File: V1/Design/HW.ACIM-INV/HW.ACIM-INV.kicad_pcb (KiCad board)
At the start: 4 copper layers, 154 x 178.5 mm, 302 parts, among them J1 AC POWER INPUT, J2 FAN, J3 MOTOR, J4 MCDBG, J8 ENCODER, M1 560V/1.75kA, M2 560V/1.75kA, M3 560V/1.75kA, M4 470V/1.2kA, M5 470V/1.2kA, M6 470V/1.2kA, M7 470V/1.2kA, Q1 20V/1A, Q10 20V/1A, Q11 20V/1A, Q2 60V/265mA, Q3 20V/1A, Q4 20V/1A, Q5 20V/1A, Q6 20V/1A, Q7 60V/265mA, Q8 60V/265mA, Q9 60V/265mA, U1 IPM 600V/15A, U10 SMPS 12V±2%/0.8A, U11 2Mbit SRAM, U12 OP-1CH, U13 LDO 3.3V±0.5%/1A, U14 SMPS 15V±2%/0.6A, U15 I=±10A, U16 I=±10A, U17 LDO 5V±0.4%/250mA, U18 OP-1CH, U19 OP-1CH, U2 OP-1CH, U20 SMPS 5V±2%/1.2A, U3 ISEN 50mV/V, U4 CMP-1CH, U5 ISEN 50mV/V, U6 ISEN 50mV/V, U7 OP-1CH, U8 OP-1CH, U9 ISO6740

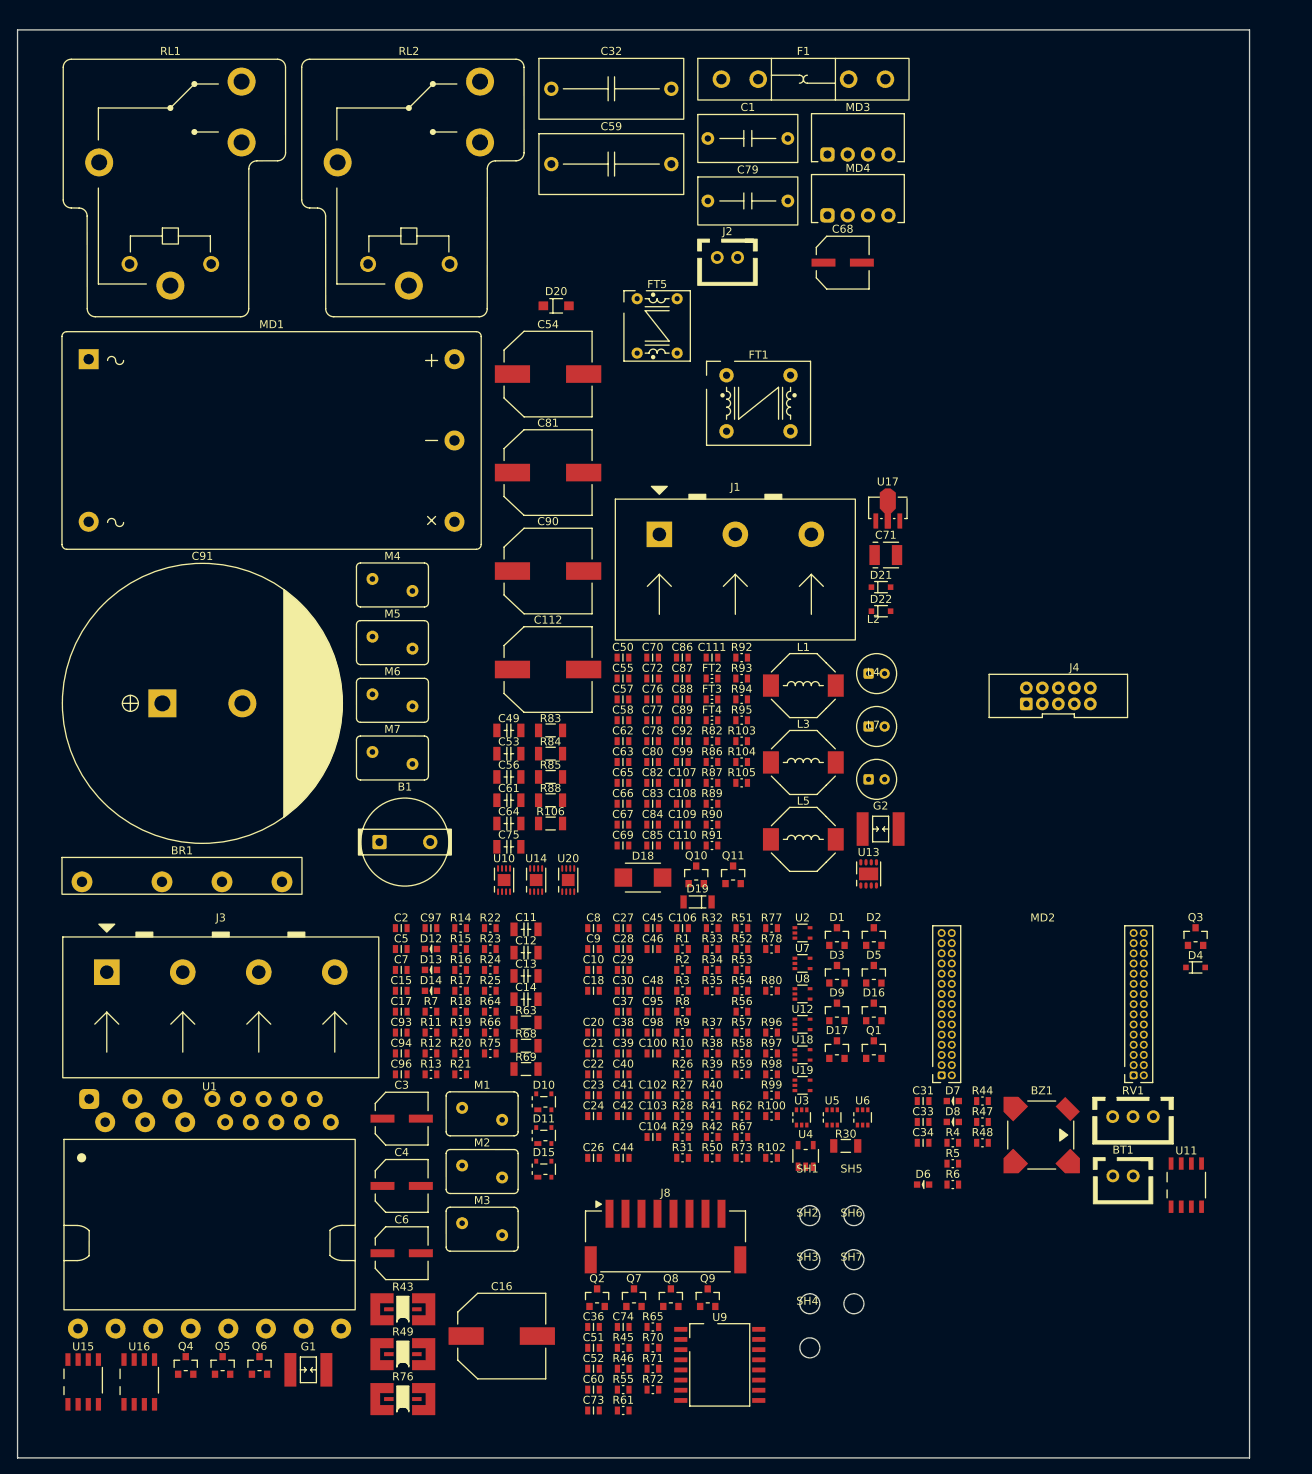
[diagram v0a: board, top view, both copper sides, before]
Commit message: V1 schematic update 17
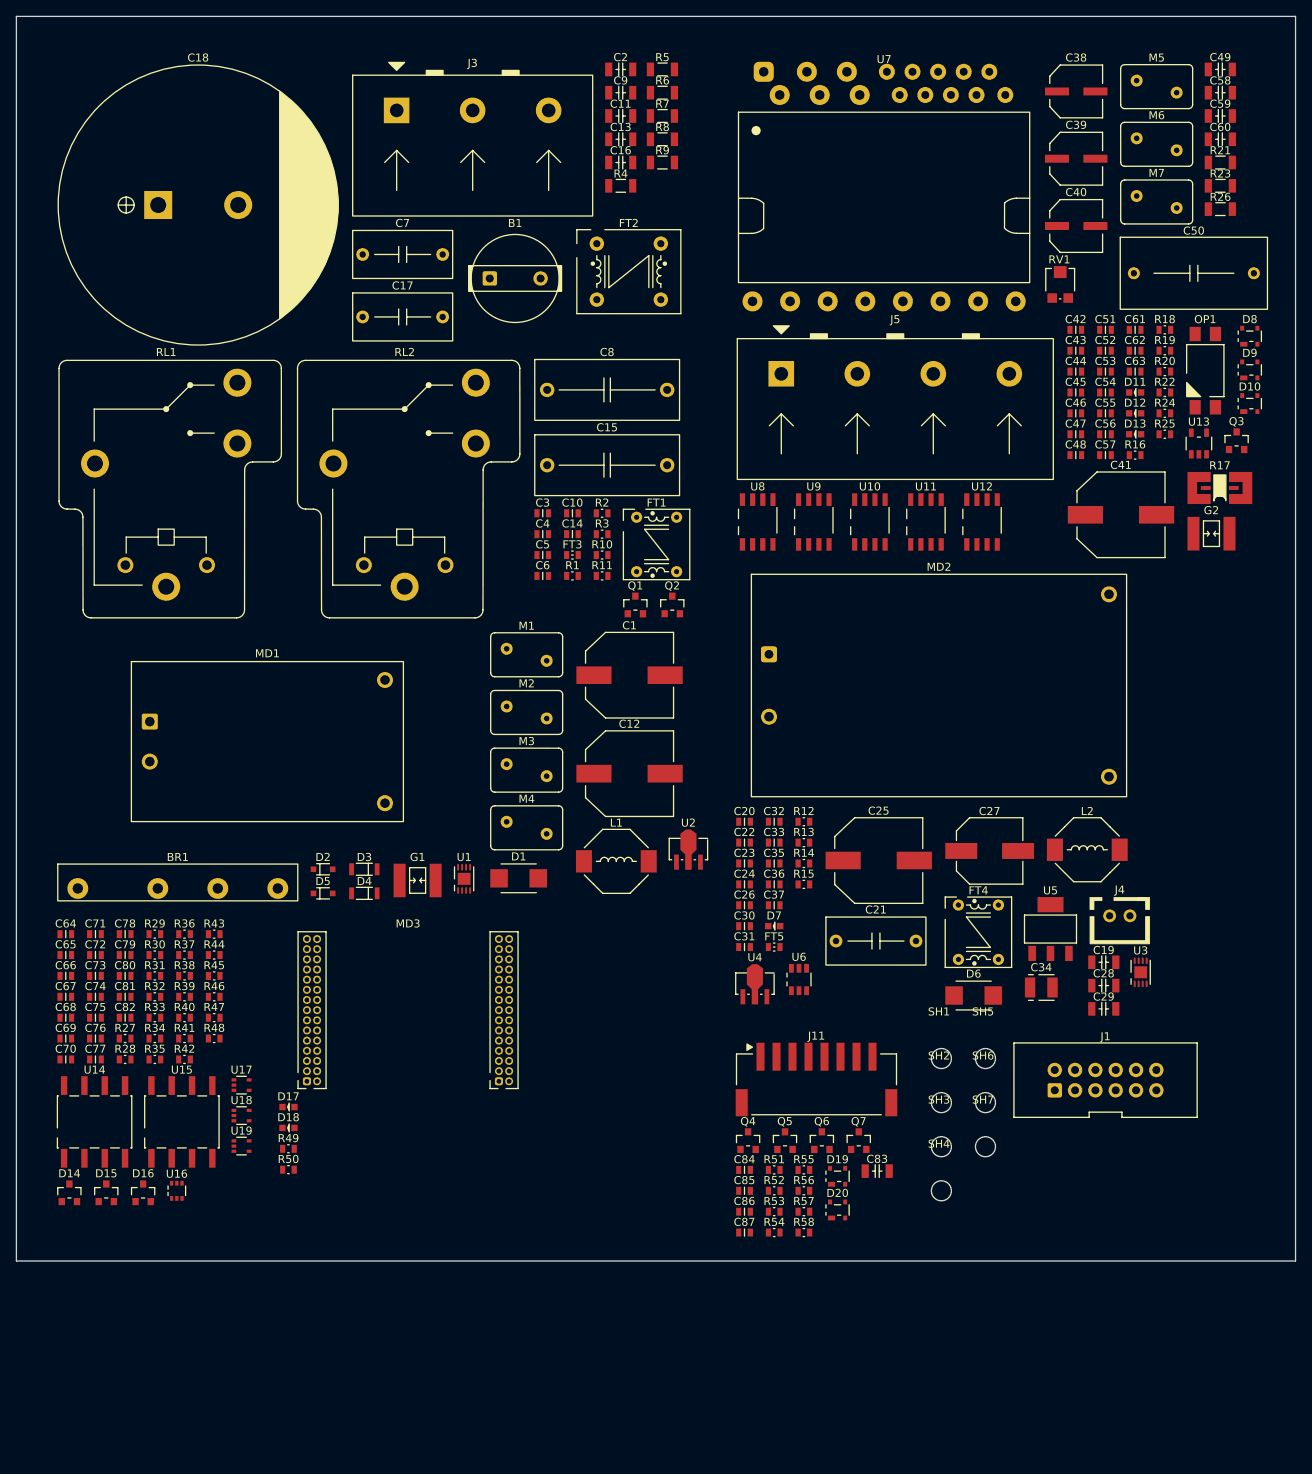
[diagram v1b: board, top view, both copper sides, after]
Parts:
- removed BT1: UBT, SAMPI:HDM-2x2.54-TH
- removed BZ1: BUZZER, SAMPI:SMT-0827-S-HT-R
- removed C100, C102, C103, C106, C94, C97, C98: 1nF, SAMPI:CAP0603
- removed C104, C109, C111, C89, C92, C93, C95, C96: 100nF, SAMPI:CAP0603
- removed C107: 10uF/35V, SAMPI:CAP0603
- removed C108, C88, C99: 10uF, SAMPI:CAP0603
- removed C110: 3.3nF, SAMPI:CAP0603
- removed C112, C90: 470uF/35V, SAMPI:CAP_ELEC-10.3x10.3-DIA10
- removed C91: 680uF/450V, SAMPI:ESMQ451VSN681MA50S
- removed D21, D22: 75V/150mA, SAMPI:SOD-323
- removed F1: 10A, SAMPI:01000056Z
- removed J2: FAN, SAMPI:HDM-2x2.54-TH
- removed J8: ENCODER, SAMPI:HDM1x8x2.0_SMA_RA
- removed L3: 22uH/1.5A, SAMPI:IND-8D43-8045
- removed L4, L7: 4.7uH/670mA, SAMPI:IND-R5-2MM-TH
- removed L5: 68uH/1A, SAMPI:IND-8D43-8045
- removed MD4: DC-DC 5V-5V/200mA, SAMPI:B1524S-1WR3
- removed Q10, Q11: 20V/1A, SAMPI:SOT23
- removed Q8, Q9: 60V/265mA, SAMPI:SOT23
- removed R100, R59, R78, R80: 10R, SAMPI:RES0603
- removed R102, R91, R95: 10K, SAMPI:RES0603
- removed R103, R62, R67, R73, R75, R82, R86, R92, R94, R96, R97, R98, R99: 100K, SAMPI:RES0603
- removed R104: 53.6K, 1%, SAMPI:RES0603
- removed R105, R90, R93: 10K, 1%, SAMPI:RES0603
- removed R106, R83, R84, R85, R88: 1M, SAMPI:RES1206
- removed R61, R65, R70, R71, R72: 4.3K, SAMPI:RES0603
- removed R63, R68, R69: 4.7R, SAMPI:RES1206
- removed R64, R66, R77: 1.1K, SAMPI:RES0603
- removed R76: 10mR/3W/1%, SAMPI:SHU2512
- removed R87: 180K, 1%, SAMPI:RES0603
- removed R89: 140K, 1%, SAMPI:RES0603
- removed U20: SMPS 5V±2%/1.2A, SAMPI:TDFN8_2x3_MCHP
- added C19: 10uF/35V, SAMPI:CAP1206, F.Cu at (150.5, 132.1)
- added C25: 470uF/35V, SAMPI:CAP_ELEC-10.3x10.3-DIA10, F.Cu at (122.4, 119.4)
- added C35: 100nF, SAMPI:CAP0603, F.Cu at (109.3, 119.8)
- added C43: 100nF, SAMPI:CAP0603, F.Cu at (147.0, 55.7)
- added C47: 10uF, SAMPI:CAP0603, F.Cu at (147.0, 66.1)
- added J11: ENCODER, SAMPI:HDM1x8x2.0_SMA_RA, F.Cu at (114.6, 146.7)
- added J5: MOTOR, SAMPI:TMB4_9.5, F.Cu at (124.5, 58.5)
- added OP1: OPTO-BJT-1CH, SAMPI:OPTO_SO4_7.6MM, F.Cu at (163.2, 58.1)
- added R36: 10R, 1%, SAMPI:RES0603, F.Cu at (35.6, 128.6)
- C1: value 100nF/400V -> 470uF/35V; footprint SAMPI:CAP_FILM_6.0x12.0x12.5-P10 -> SAMPI:CAP_ELEC-10.3x10.3-DIA10
- C10: value 1nF -> 100nF
- C12: value 100pF/2kV -> 470uF/25V; footprint SAMPI:CAP1206 -> SAMPI:CAP_ELEC-10.3x10.3-DIA10
- C14, C53: value 100pF/2kV -> 10uF; footprint SAMPI:CAP1206 -> SAMPI:CAP0603
- C15: value 22pF -> 1uF/400V; footprint SAMPI:CAP0603 -> SAMPI:ECWFE2W105
- C16: value 470uF -> 100pF/2kV; footprint SAMPI:CAP_ELEC-10.3x10.3-DIA10 -> SAMPI:CAP1206
- C17, C7: value 100nF -> 100nF/400V; footprint SAMPI:CAP0603 -> SAMPI:CAP_FILM_6.0x12.0x12.5-P10
- C18: value 1nF -> 680uF/450V; footprint SAMPI:CAP0603 -> SAMPI:ESMQ451VSN681MA50S
- C2, C28, C29: value 100nF -> 10uF/35V; footprint SAMPI:CAP0603 -> SAMPI:CAP1206
- C20, C46, C48: value 100nF -> 10uF
- C21: value 1nF -> 100nF/400V; footprint SAMPI:CAP0603 -> SAMPI:CAP_FILM_6.0x12.0x12.5-P10
- C23: value 100nF -> 3.3nF
- C27: value 100nF -> 470uF/16V; footprint SAMPI:CAP0603 -> SAMPI:CAP_ELEC-8.3x8.3-DIA8.0
- C3: value 47uF/35V -> 10uF; footprint SAMPI:CAP_ELEC-6.6x6.6-DIA6.3 -> SAMPI:CAP0603
- C30, C31, C37: value 1nF -> 10uF
- C32: value 1uF/400V -> 100nF; footprint SAMPI:ECWFE2W105 -> SAMPI:CAP0603
- C34: value 100nF -> 220uF/6.3V; footprint SAMPI:CAP0603 -> SAMPI:CAP1411
- C36, C51: value 22pF -> 100nF
- C38, C40: value 100nF -> 47uF/35V; footprint SAMPI:CAP0603 -> SAMPI:CAP_ELEC-6.6x6.6-DIA6.3
- C39: value 1nF -> 47uF/35V; footprint SAMPI:CAP0603 -> SAMPI:CAP_ELEC-6.6x6.6-DIA6.3
- C4, C68: value 47uF/35V -> 100nF; footprint SAMPI:CAP_ELEC-6.6x6.6-DIA6.3 -> SAMPI:CAP0603
- C41: value 100nF -> 470uF/25V; footprint SAMPI:CAP0603 -> SAMPI:CAP_ELEC-10.3x10.3-DIA10
- C50: value 100nF -> 470nF/630V; footprint SAMPI:CAP0603 -> SAMPI:FCAP-15MM
- C52: value 22pF -> 1nF
- C54: value 470uF/35V -> 10uF; footprint SAMPI:CAP_ELEC-10.3x10.3-DIA10 -> SAMPI:CAP0603
- C56, C61: value 100pF/2kV -> 100nF; footprint SAMPI:CAP1206 -> SAMPI:CAP0603
- C57, C74: value 10uF -> 1nF
- C58, C9: value 100nF -> 100pF/2kV; footprint SAMPI:CAP0603 -> SAMPI:CAP1206
- C59: value 1uF/400V -> 100pF/2kV; footprint SAMPI:ECWFE2W105 -> SAMPI:CAP1206
- C6: value 47uF/35V -> 3.3nF; footprint SAMPI:CAP_ELEC-6.6x6.6-DIA6.3 -> SAMPI:CAP0603
- C60: value 22pF -> 100pF/2kV; footprint SAMPI:CAP0603 -> SAMPI:CAP1206
- C62: value 10uF/35V -> 100nF
- C64, C75: value 100pF/2kV -> 1nF; footprint SAMPI:CAP1206 -> SAMPI:CAP0603
- C65, C76, C77, C78: value 100nF -> 1nF
- C66: value 3.3nF -> 100nF
- C70, C82: value 10uF/35V -> 1nF
- C71: value 220uF/6.3V -> 1nF; footprint SAMPI:CAP1411 -> SAMPI:CAP0603
- C72, C73, C80: value 10uF -> 100nF
- C79: value 100nF/400V -> 100nF; footprint SAMPI:CAP_FILM_6.0x12.0x12.5-P10 -> SAMPI:CAP0603
- C8: value 1nF -> 1uF/400V; footprint SAMPI:CAP0603 -> SAMPI:ECWFE2W105
- C81: value 470uF/35V -> 1nF; footprint SAMPI:CAP_ELEC-10.3x10.3-DIA10 -> SAMPI:CAP0603
- C83: value 10uF -> 10uF/35V; footprint SAMPI:CAP0603 -> SAMPI:CAP1206
- C84: value 100nF -> 22pF
- C85: value 3.3nF -> 22pF
- D1: value GP DIODE -> 24V; footprint SAMPI:SOT23 -> SAMPI:DO-214AA-12
- D10: value TVS 5.5V 3-CH -> TVS 5.5V
- D11: value TVS 5.5V 3-CH -> PV; footprint SAMPI:SOT143B_NEXT -> SAMPI:LED0603
- D12: value PU -> PW
- D13: value PV -> PU
- D14: value PW -> GP DIODE; footprint SAMPI:LED0603 -> SAMPI:SOT23
- D15: value TVS 5.5V 3-CH -> GP DIODE; footprint SAMPI:SOT143B_NEXT -> SAMPI:SOT23
- D17: value GP DIODE -> ERR; footprint SAMPI:SOT23 -> SAMPI:LED0603
- D18: value 24V -> RUN; footprint SAMPI:DO-214AA-12 -> SAMPI:LED0603
- D19: value 24V -> TVS 5.5V; footprint SAMPI:SOD-80C_DO-213AC -> SAMPI:SOT143B_NEXT
- D2, D5: value GP DIODE -> 75V/150mA; footprint SAMPI:SOT23 -> SAMPI:SOD-323
- D20: value 5.1V -> TVS 5.5V; footprint Liem:SOD-123 -> SAMPI:SOT143B_NEXT
- D3: value GP DIODE -> 6V2; footprint SAMPI:SOT23 -> SAMPI:SOD80C-LL34
- D4: value 75V/150mA -> 6V2; footprint SAMPI:SOD-323 -> SAMPI:SOD80C-LL34
- D6: value ERR -> 24V; footprint SAMPI:LED0603 -> SAMPI:DO-214AA-12
- D7: value RUN -> PWR
- D8: value PWR -> TVS 5.5V; footprint SAMPI:LED0603 -> SAMPI:SOT143B_NEXT
- D9: value GP DIODE -> TVS 5.5V; footprint SAMPI:SOT23 -> SAMPI:SOT143B_NEXT
- FT1: value 5mH/2.5A -> 15mH/500mA; footprint SAMPI:IND-SQ1010 -> SAMPI:EE8.3
- FT2: value 120R@100MHz -> 5mH/2.5A; footprint SAMPI:FT0603 -> SAMPI:IND-SQ1010
- FT4: value 120R@100MHz -> 15mH/500mA; footprint SAMPI:FT0603 -> SAMPI:EE8.3
- FT5: value 15mH/500mA -> 120R@100MHz; footprint SAMPI:EE8.3 -> SAMPI:FT0603
- J1: value AC POWER INPUT -> MCDBG; footprint SAMPI:TMB3_9.5 -> SAMPI:IDC-2x6x2.54MM_TH
- J3: value MOTOR -> AC POWER INPUT; footprint SAMPI:TMB4_9.5 -> SAMPI:TMB3_9.5
- J4: value MCDBG -> FAN; footprint SAMPI:IDC-2x5x2MM-TH -> SAMPI:HDM-2x2.54-TH
- L1: value 56uH/1A -> 68uH/1A
- L2: value 4.7uH/670mA -> 56uH/1A; footprint SAMPI:IND-R5-2MM-TH -> SAMPI:IND-8D43-8045
- M1, M2, M3: value 560V/1.75kA -> 470V/1.2kA
- M5, M6, M7: value 470V/1.2kA -> 560V/1.75kA
- MD1: value AC-DC 24V±2%/10W -> 24V±2%/3W; footprint SAMPI:LD10-23BxxR2-RC -> SAMPI:HLK-PMxx
- MD2: value ACIM-MCU -> 24V±2%/10W; footprint SAMPI:HW.ACIM-MCU -> SAMPI:HLK-10M
- MD3: value DC-DC 15V/24V-24V/42mA -> ACIM-MCU; footprint SAMPI:B1524S-1WR3 -> SAMPI:HW.ACIM-MCU
- Q2: value 60V/265mA -> 20V/1A
- Q4, Q5, Q6: value 20V/1A -> 60V/265mA
- R1: value 10R -> 10K
- R10, R11, R22: value 1.1K -> 10K
- R12, R16: value 100K -> 10K
- R13: value 1.1K -> 140K, 1%
- R14: value 1.1K -> 10K, 1%
- R15, R19, R20: value 1.1K -> 1K
- R17: value 100K -> 10mR/3W/1%; footprint SAMPI:RES0603 -> SAMPI:SHU2512
- R18, R24: value 100K -> 1K
- R2: value 10R -> 191K, 1%
- R21: value 1.1K -> 4.7R; footprint SAMPI:RES0603 -> SAMPI:RES1206
- R23, R26: value 100K -> 4.7R; footprint SAMPI:RES0603 -> SAMPI:RES1206
- R25: value 100K -> 1.2M
- R27: value 10R -> 100K, 1%
- R28: value 100K -> 100K, 1%
- R29, R44: value 1.1K -> 100K, 1%
- R3: value 5.2K -> 10K, 1%
- R30: value 1M -> 1.1K, 1%; footprint SAMPI:RES1206 -> SAMPI:RES0603
- R31: value 470K -> 10R, 1%
- R32, R41: value 10R -> 10R, 1%
- R33, R47: value 1.1K -> 10R, 1%
- R34, R35: value 100K -> 10R, 1%
- R37: value 100K -> 10K, 1%
- R38: value 10R -> 10K, 1%
- R39: value 1.1K -> 4.99K, 1%
- R4: value 10R -> 1M; footprint SAMPI:RES0603 -> SAMPI:RES1206
- R40: value 10R -> 4.99K, 1%
- R42: value 5.2K -> 10R, 1%
- R43: value 10mR/3W/1% -> 100K, 1%; footprint SAMPI:SHU2512 -> SAMPI:RES0603
- R45, R46: value 4.3K -> 100K, 1%
- R48: value 10K -> 10R, 1%
- R49: value 10mR/3W/1% -> 1K; footprint SAMPI:SHU2512 -> SAMPI:RES0603
- R5, R7: value 1.1K -> 1M; footprint SAMPI:RES0603 -> SAMPI:RES1206
- R50: value 10R -> 1K
- R51, R52: value 10R -> 2.2K
- R53, R56, R57: value 100K -> 2.2K
- R54: value 10K -> 2.2K
- R55: value 4.3K -> 2.2K
- R58: value 1.1K -> 2.2K
- R6, R8, R9: value 100K -> 1M; footprint SAMPI:RES0603 -> SAMPI:RES1206
- RV1: value 10K -> 20K; footprint Liem:HDM-3x2.54-TH -> SAMPI:TC33X-2
- U1: value IPM 600V/15A -> SMPS 16V±2%/0.6A; footprint SAMPI:CIPOS-MINI -> SAMPI:TDFN8_2x3_MCHP
- U10: value SMPS 12V±2%/0.8A -> DIGI ISO; footprint SAMPI:TDFN8_2x3_MCHP -> SAMPI:SOIC8_ALL
- U11: value 2Mbit SRAM -> I=±10A; footprint SAMPI:SOIC8_3.9_MCHP -> SAMPI:SOIC8_ALL
- U12: value OP-1CH -> I=±10A; footprint SAMPI:SOT353 -> SAMPI:SOIC8_ALL
- U13: value LDO 3.3V±0.5%/1A -> CMP-1CH; footprint SAMPI:DFN8_3x3_MCHP -> SAMPI:SOT25_DIODES
- U14: value SMPS 15V±2%/0.6A -> ISO OPAMP 1-CH; footprint SAMPI:TDFN8_2x3_MCHP -> SAMPI:SOP8-2.54
- U15: value I=±10A -> ISO OPAMP 1-CH; footprint SAMPI:SOIC8_ALL -> SAMPI:SOP8-2.54
- U16: value I=±10A -> ISEN 50mV/V; footprint SAMPI:SOIC8_ALL -> SAMPI:SOT363
- U17: value LDO 5V±0.4%/250mA -> OP-1CH; footprint SAMPI:SOT-89 -> SAMPI:SOT353
- U2: value OP-1CH -> LDO 5V±1%; footprint SAMPI:SOT353 -> SAMPI:SOT-89
- U3: value ISEN 50mV/V -> SMPS 12V±2%/0.8A; footprint SAMPI:SOT363 -> SAMPI:TDFN8_2x3_MCHP
- U4: value CMP-1CH -> LDO 5V±1%; footprint SAMPI:SOT25_DIODES -> SAMPI:SOT-89
- U5: value ISEN 50mV/V -> LDO 3V3±2%; footprint SAMPI:SOT363 -> SAMPI:SOT-223-3
- U6: value ISEN 50mV/V -> LDO 3.3V±0.1%/20mA; footprint SAMPI:SOT363 -> SAMPI:SOT-23-6_MCHP
- U7: value OP-1CH -> IPM 600V/15A; footprint SAMPI:SOT353 -> SAMPI:CIPOS-MINI
- U8: value OP-1CH -> DIGI ISO; footprint SAMPI:SOT353 -> SAMPI:SOIC8_ALL
- U9: value ISO6740 -> DIGI ISO; footprint SAMPI:SOIC16-W -> SAMPI:SOIC8_ALL
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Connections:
- B1 pad 1: Net-(RL1-NC) -> Net-(RL2-NC)
- C10 pad 1: AGND -> GND_INV
- C10 pad 2: /MCU/MC_ALT_IU_SEN -> +16V_INV
- C11 pad 2: /Inverter/MC_UW -> CHASSIS
- C13 pad 1: /Inverter/MC_UU -> AC1
- C13 pad 2: Net-(C13-Pad2) -> CHASSIS
- C14 pad 1: VDC -> GND_INV
- C14 pad 2: PGND -> +5V_INV
- C15 pad 1: AGND -> AC2
- C15 pad 2: /Inverter/MC_TEMP_SEN -> AC1
- C17 pad 1: +15V -> PGND
- C17 pad 2: GND -> VDC
- C2 pad 1: Net-(U1-VBU) -> GND_INV
- C2 pad 2: Net-(U1-VSU) -> +24V_INV
- C20 pad 1: /MCU/MC_UU_DIV -> GND_MCU
- C20 pad 2: AGND -> Net-(U3-VCC)
- C21 pad 1: GND -> Net-(MD2-ACN)
- C21 pad 2: /MCU/~{MC_PWM_FLT} -> Net-(MD2-ACL)
- C22 pad 1: AGND -> Net-(U3-SW)
- C22 pad 2: Net-(C22-Pad2) -> Net-(U3-BOOST)
- C23 pad 1: Net-(D2-COM) -> Net-(U3-VFB)
- C23 pad 2: AGND -> +12V_MCU
- C24 pad 1: AGND -> GND_MCU
- C24 pad 2: AVDD -> +24V_MCU
- C26 pad 1: /MCU/MC_UV_DIV -> GND_MCU
- C26 pad 2: AGND -> +12V_MCU
- C28 pad 1: Net-(D3-COM) -> GND_MCU
- C28 pad 2: AGND -> +12V_MCU
- C29 pad 1: GND -> GND_MCU
- C29 pad 2: VREF -> +12V_MCU
- C30 pad 1: AGND -> GND_MCU
- C30 pad 2: /MCU/MC_IV_SEN -> +5V_MCU
- C31 pad 1: AGND -> GND_MCU
- C31 pad 2: /MCU/MC_VR_DIV -> +5V_MCU
- C32 pad 1: Net-(C32-Pad1) -> GND_MCU
- C32 pad 2: Net-(C32-Pad2) -> +3V3_MCU
- C33 pad 1: GND -> GND_MCU
- C33 pad 2: /MCU/~{BT_UBT} -> +5V_MCU
- C36 pad 1: GND -> GND_ADC
- C36 pad 2: /ENCODER/ENC_HOME -> +3V3_ADC
- C37 pad 1: Net-(D9-COM) -> GND_ADC
- C37 pad 2: Net-(D9-A1) -> +3V3_ADC
- C42 pad 1: AGND -> +16V_INV
- C42 pad 2: AVDD -> GND_INV
- C44 pad 1: /MCU/MC_UW_DIV -> Net-(U7-VBV)
- C44 pad 2: AGND -> Net-(U7-VSV)
- C45 pad 1: Net-(D17-COM) -> Net-(U7-VBW)
- C45 pad 2: AGND -> Net-(U7-VSW)
- C46 pad 1: AGND -> GND_INV
- C46 pad 2: AVDD -> +5V_INV
- C48 pad 1: /MCU/MC_UDC_DIV -> GND_INV
- C48 pad 2: AGND -> +5V_INV
- C49 pad 1: Net-(C32-Pad1) -> VDC
- C49 pad 2: CHASSIS -> PGND
- C5 pad 1: Net-(U1-VBV) -> Net-(U1-SW)
- C5 pad 2: Net-(U1-VSV) -> Net-(U1-BOOST)
- C50 pad 1: GND -> VDC
- C50 pad 2: +24V -> PGND
- C51 pad 1: GND -> GND_MCU
- C51 pad 2: /ENCODER/ENC_A -> +5V_MCU
- C52 pad 1: GND -> GND_MCU
- C52 pad 2: /ENCODER/ENC_B -> Net-(U11-FILTER)
- C53 pad 1: Net-(C32-Pad2) -> GND_MCU
- C53 pad 2: CHASSIS -> +3V3_MCU
- C55 pad 1: GND -> GND_MCU
- C55 pad 2: Net-(MD4-VI+) -> +3V3_MCU
- C56 pad 1: AC1 -> GND_MCU
- C56 pad 2: CHASSIS -> +5V_MCU
- C57 pad 1: GND -> GND_MCU
- C57 pad 2: Net-(U10-VCC) -> Net-(U12-FILTER)
- C58 pad 1: GND -> /INVERTER/MC_U
- C58 pad 2: +15V -> Net-(C58-Pad2)
- C59 pad 1: AC2 -> Net-(C59-Pad1)
- C59 pad 2: AC1 -> /INVERTER/MC_V
- C60 pad 1: GND -> /INVERTER/MC_W
- C60 pad 2: /ENCODER/ENC_INDEX -> Net-(C60-Pad2)
- C61 pad 1: AC2 -> GND_INV
- C61 pad 2: CHASSIS -> +5V_INV
- C62 pad 1: GND -> GND_INV
- C62 pad 2: Net-(MD3-VI+) -> Net-(RV1-WIPER)
- C63 pad 1: Net-(U10-SW) -> GND_INV
- C63 pad 2: Net-(U10-BOOST) -> /INVERTER/IPM_TEMP_SEN
- C64 pad 1: GND -> Net-(D15-COM)
- C64 pad 2: GND1 -> Net-(D15-A1)
- C65 pad 1: GND -> Net-(D16-COM)
- C65 pad 2: +5V -> Net-(D16-A1)
- C66 pad 1: Net-(U10-VFB) -> +5V_INV
- C66 pad 2: +12V -> GND_INV
- C67 pad 1: GND1 -> +5V_INV
- C67 pad 2: +24V_ISO -> GND_INV
- C69 pad 1: GND -> +5V_MCU
- C69 pad 2: +12V -> GND_MCU
- C7 pad 1: Net-(U1-VBW) -> Net-(MD1-ACN)
- C7 pad 2: Net-(U1-VSW) -> Net-(MD1-ACL)
- C70 pad 1: GND -> Net-(U16-IN-)
- C70 pad 2: +24V -> Net-(U16-IN+)
- C72 pad 1: GND -> GND_MCU
- C72 pad 2: +5V -> +5V_MCU
- C73 pad 1: GND_ISO -> GND_MCU
- C73 pad 2: +5V_ISO -> +5V_MCU
- C74 pad 1: GND -> GND_ADC
- C74 pad 2: +3V3 -> /MCU/MC_UDC_DIV
- C75 pad 1: GND -> GND_ADC
- C75 pad 2: GND1 -> Net-(U16-OUT)
- C76 pad 1: GND1 -> GND_ADC
- C76 pad 2: +5V_ISO -> /MCU/MC_IDC_SEN
- C77 pad 1: GND -> GND_MCU
- C77 pad 2: Net-(U13-CDELAY) -> Net-(U18-IN+)
- C78 pad 1: GND -> GND_MCU
- C78 pad 2: +3V3 -> Net-(U19-IN+)
- C79 pad 1: PGND -> GND_MCU
- C79 pad 2: VDC -> +5V_MCU
- C8 pad 1: Net-(D1-COM) -> Net-(C8-Pad1)
- C8 pad 2: Net-(D1-A1) -> Net-(C11-Pad1)
- C80 pad 1: GND1 -> GND_MCU
- C80 pad 2: +5V_ISO -> +5V_MCU
- C82 pad 1: GND -> GND_ADC
- C82 pad 2: +24V -> /MCU/MC_IV_SEN
- C83 pad 1: GND -> GND_MCU
- C83 pad 2: Net-(U14-VCC) -> /ENCODER/V_ENC
- C84 pad 1: Net-(U14-SW) -> GND_MCU
- C84 pad 2: Net-(U14-BOOST) -> /ENCODER/ENC_HOME
- C85 pad 1: Net-(U14-VFB) -> GND_MCU
- C85 pad 2: +15V -> /ENCODER/ENC_INDEX
- C86 pad 1: GND -> GND_MCU
- C86 pad 2: +3V3 -> /ENCODER/ENC_B
- C87 pad 1: AGND -> GND_MCU
- C87 pad 2: AVDD -> /ENCODER/ENC_A
- C9 pad 1: GND -> Net-(C8-Pad1)
- C9 pad 2: VREF -> CHASSIS
- D1 pad 1: Net-(D1-A1) -> GND_INV
- D1 pad 2: Net-(D1-A1) -> +24V_INV
- D10 pad 1: GND -> GND_INV
- D10 pad 2: /Inverter/MC_PWM_UH -> /INVERTER/IPM_PWM_WH
- D10 pad 3: /Inverter/MC_PWM_VH -> /INVERTER/IPM_PWM_WL
- D10 pad 4: +3V3 -> +5V_INV
- D12 pad K: Net-(Q4-D) -> GND_MCU
- D13 pad K: Net-(Q5-D) -> GND_MCU
- D15 pad 1: GND -> Net-(D15-A1)
- D15 pad 2: /Inverter/MC_PWM_WL -> Net-(D15-A1)
- D15 pad 3: /Inverter/MC_PWM_WH -> Net-(D15-COM)
- D16 pad 1: AGND -> Net-(D16-A1)
- D16 pad 2: AVDD -> Net-(D16-A1)
- D4 pad A: Net-(BZ1-V-) -> Net-(Q2-D)
- D4 pad K: +5V -> Net-(RL2-COIL1)
- D7 pad A: /MCU/IND_RUN -> Net-(D7-PadA)
- D7 pad K: Net-(D7-PadK) -> GND_MCU
- D9 pad 1: Net-(D9-A1) -> GND_INV
- D9 pad 2: Net-(D9-A1) -> /INVERTER/IPM_PWM_VH
- D9 pad 3: Net-(D9-COM) -> /INVERTER/IPM_PWM_VL
- FT1 pad 1: Net-(C32-Pad1) -> AC2
- FT1 pad 2: AC2 -> Net-(MD1-ACN)
- FT1 pad 3: Net-(C32-Pad2) -> AC1
- FT1 pad 4: AC1 -> Net-(MD1-ACL)
- FT2 pad 1: AGND -> Net-(C8-Pad1)
- FT2 pad 2: GND -> AC2
- FT3 pad 1: GND -> GND_INV
- FT4 pad 1: +3V3 -> AC2
- FT4 pad 2: AVDD -> Net-(MD2-ACN)
- FT5 pad 1: AC2 -> GND_MCU
- FT5 pad 2: Net-(MD1-ACN) -> GND_ADC
- G2 pad 1: CHASSIS -> Net-(G2-Pad1)
- G2 pad 2: Net-(G2-Pad2) -> CHASSIS
- J1 pad 1: CHASSIS -> /MCU/DB_TXD
- J1 pad 2: Net-(C32-Pad1) -> /MCU/~{MCLR}
- J1 pad 3: Net-(F1-Pad1) -> /MCU/DB_RXD
- J3 pad 1: Net-(G1-Pad2) -> CHASSIS
- J3 pad 2: /Inverter/MC_UV -> Net-(C8-Pad1)
- J3 pad 3: /Inverter/MC_UW -> Net-(C11-Pad1)
- J4 pad 1: /MCU/DV_TXD -> +12V_MCU
- J4 pad 2: /MCU/~{MCLR} -> GND
- L1 pad 1: Net-(U10-SW) -> Net-(U1-SW)
- L1 pad 2: +12V -> +16V_INV
- L2 pad 1: +15V -> Net-(U3-SW)
- L2 pad 2: Net-(MD3-VI+) -> +12V_MCU
- M1 pad 1: Net-(G1-Pad2) -> Net-(C8-Pad1)
- M1 pad 2: /Inverter/MC_UV -> Net-(C11-Pad1)
- M2 pad 2: /Inverter/MC_UW -> Net-(C8-Pad1)
- M3 pad 2: /Inverter/MC_UU -> Net-(C11-Pad1)
- M4 pad 1: Net-(C32-Pad1) -> AC2
- M4 pad 2: Net-(C32-Pad2) -> AC1
- M5 pad 1: Net-(G2-Pad2) -> Net-(G2-Pad1)
- M5 pad 2: Net-(C32-Pad1) -> /INVERTER/MC_U
- M6 pad 1: Net-(G2-Pad2) -> Net-(G2-Pad1)
- M6 pad 2: Net-(C32-Pad2) -> /INVERTER/MC_V
- M7 pad 1: AC2 -> Net-(G2-Pad1)
- M7 pad 2: AC1 -> /INVERTER/MC_W
- MD1 pad 3: unconnected-(MD1-NC-Pad3) -> GND_INV
- MD1 pad 4: GND -> +24V_INV
- Q1 pad 1: /MCU/~{MC_PWM_FLT} -> /INVERTER POWER/PWR_RELAY
- Q1 pad 2: GND -> GND_MCU
- Q1 pad 3: /Inverter/MC_PWM_FLT -> Net-(Q1-D)
- Q2 pad 1: +5V_ISO -> /INVERTER POWER/~{DEV_RELAY}
- Q2 pad 2: Net-(Q2-S) -> GND_MCU
- Q2 pad 3: /ENCODER/HOME -> Net-(Q2-D)
- Q3 pad 1: /MCU/IND_ERR -> /INVERTER/IPM_PWM_FLT
- Q3 pad 2: GND -> GND_INV
- Q3 pad 3: Net-(BZ1-V-) -> Net-(OP1-K)
- Q4 pad 1: /Inverter/IPM_PWM_UL -> +3V3_MCU
- Q4 pad 2: GND -> /ENCODER/ENC_HOME
- Q4 pad 3: Net-(Q4-D) -> /ENCODER/HOME
- Q5 pad 1: /Inverter/IPM_PWM_VL -> +3V3_MCU
- Q5 pad 2: GND -> /ENCODER/ENC_INDEX
- Q5 pad 3: Net-(Q5-D) -> /ENCODER/INDEX
- Q6 pad 1: /Inverter/IPM_PWM_WL -> +3V3_MCU
- Q6 pad 2: GND -> /ENCODER/ENC_B
- Q6 pad 3: Net-(Q6-D) -> /ENCODER/PULSE_B
- Q7 pad 1: +5V_ISO -> +3V3_MCU
- Q7 pad 2: Net-(Q7-S) -> /ENCODER/ENC_A
- Q7 pad 3: /ENCODER/INDEX -> /ENCODER/PULSE_A
- R1 pad 1: Net-(D1-A1) -> Net-(U1-EN)
- R1 pad 2: /Inverter/MC_IU_SEN_P -> +24V_INV
- R10 pad 1: Net-(U4-VIN-) -> /INVERTER POWER/PWR_RELAY
- R10 pad 2: /MCU/MC_IDC_SEN -> GND_MCU
- R11 pad 1: Net-(U1-VFO) -> /INVERTER POWER/~{DEV_RELAY}
- R11 pad 2: /Inverter/MC_TEMP_SEN -> GND_MCU
- R12 pad 1: AVDD -> Net-(U3-EN)
- R12 pad 2: Net-(U1-VFO) -> +24V_MCU
- R13 pad 1: /Inverter/IPM_PWM_UH -> Net-(U3-VFB)
- R13 pad 2: /Inverter/MC_PWM_UH -> +12V_MCU
- R14 pad 1: /Inverter/IPM_PWM_VH -> GND_MCU
- R14 pad 2: /Inverter/MC_PWM_VH -> Net-(U3-VFB)
- R15 pad 1: /Inverter/IPM_PWM_WH -> +3V3_MCU
- R15 pad 2: /Inverter/MC_PWM_WH -> Net-(D7-PadA)
- R16 pad 1: GND -> +5V_INV
- R16 pad 2: /Inverter/IPM_PWM_WH -> /INVERTER/IPM_TEMP_SEN
- R17 pad 1: GND -> PGND
- R17 pad 2: /Inverter/IPM_PWM_VH -> Net-(U7-NU)
- R18 pad 1: GND -> Net-(D13-PadA)
- R18 pad 2: /Inverter/IPM_PWM_UH -> /INVERTER/MC_PWM_UH
- R19 pad 1: /Inverter/IPM_PWM_UL -> Net-(D11-PadA)
- R19 pad 2: /Inverter/MC_PWM_UL -> /INVERTER/MC_PWM_VH
- R2 pad 1: Net-(D1-COM) -> Net-(U1-VFB)
- R2 pad 2: /Inverter/MC_IU_SEN_N -> +16V_INV
- R20 pad 2: +3V3 -> /INVERTER/MC_PWM_WH
- R21 pad 1: /Inverter/IPM_PWM_VL -> Net-(C58-Pad2)
- R21 pad 2: /Inverter/MC_PWM_VL -> /INVERTER/MC_V
- R22 pad 1: /Inverter/IPM_PWM_WL -> +3V3_MCU
- R22 pad 2: /Inverter/MC_PWM_WL -> /INVERTER/MC_TEMP_FLT
- R23 pad 1: GND -> Net-(C59-Pad1)
- R23 pad 2: /Inverter/IPM_PWM_WL -> /INVERTER/MC_W
- R24 pad 1: GND -> Net-(OP1-A)
- R24 pad 2: /Inverter/IPM_PWM_VL -> +5V_INV
- R25 pad 1: GND -> /INVERTER/IPM_TEMP_SEN
- R25 pad 2: /Inverter/IPM_PWM_UL -> /INVERTER/IPM_PWM_FLT
- R26 pad 1: Net-(R26-Pad1) -> Net-(C60-Pad2)
- R26 pad 2: Net-(D2-COM) -> /INVERTER/MC_U
- R27 pad 1: Net-(U4-VOUT) -> VDC
- R27 pad 2: /MCU/~{MC_PWM_FLT} -> Net-(R27-Pad2)
- R28 pad 1: Net-(C22-Pad2) -> Net-(R27-Pad2)
- R28 pad 2: AVDD -> Net-(R28-Pad2)
- R29 pad 1: Net-(U4-VIN+) -> Net-(R28-Pad2)
- R29 pad 2: Net-(C22-Pad2) -> Net-(D14-COM)
- R3 pad 1: Net-(U5-OUT) -> GND_INV
- R3 pad 2: /MCU/MC_IU_SEN -> Net-(U1-VFB)
- R30 pad 1: Net-(U4-VOUT) -> Net-(D14-COM)
- R30 pad 2: Net-(U4-VIN+) -> GND_INV
- R31 pad 1: AGND -> Net-(D15-A1)
- R31 pad 2: Net-(C22-Pad2) -> /INVERTER/MC_IDC_P
- R32 pad 1: /MCU/MC_UU_DIV -> Net-(D15-COM)
- R32 pad 2: Net-(U2-IN-) -> /INVERTER/MC_IDC_N
- R33 pad 1: Net-(D2-COM) -> Net-(D16-A1)
- R33 pad 2: AGND -> Net-(D14-COM)
- R34 pad 1: /Inverter/MC_UV -> Net-(D16-COM)
- R34 pad 2: Net-(R34-Pad2) -> GND_INV
- R35 pad 1: Net-(R34-Pad2) -> Net-(U16-IN+)
- R35 pad 2: Net-(R35-Pad2) -> Net-(U14-VOUT+)
- R37 pad 1: Net-(R35-Pad2) -> Net-(U17-IN+)
- R37 pad 2: Net-(D3-COM) -> Net-(U15-VOUT+)
- R38 pad 1: /MCU/MC_UV_DIV -> Net-(U17-IN-)
- R38 pad 2: Net-(U12-IN-) -> Net-(U15-VOUT-)
- R39 pad 1: Net-(D3-COM) -> Net-(U17-IN+)
- R39 pad 2: AGND -> GND_MCU
- R4 pad 1: Net-(RV1-WIPER) -> Net-(R4-Pad1)
- R4 pad 2: /MCU/MC_VR_DIV -> AC1
- R40 pad 1: Net-(D5-A1) -> Net-(U17-IN-)
- R40 pad 2: /Inverter/MC_IV_SEN_P -> Net-(U17-OUT)
- R41 pad 1: Net-(D5-COM) -> /MCU/MC_UDC_DIV
- R41 pad 2: /Inverter/MC_IV_SEN_N -> Net-(U17-OUT)
- R42 pad 1: Net-(U3-OUT) -> Net-(U16-OUT)
- R42 pad 2: /MCU/MC_IV_SEN -> /MCU/MC_IDC_SEN
- R43 pad 1: Net-(U1-NW) -> /INVERTER/MC_IU_HAL
- R43 pad 2: Net-(U1-NV) -> Net-(U18-IN+)
- R44 pad 1: Net-(D7-PadK) -> Net-(U18-IN+)
- R44 pad 2: GND -> GND_MCU
- R45 pad 1: +24V_ISO -> /INVERTER/MC_IV_HAL
- R45 pad 2: /ENCODER/INDEX -> Net-(U19-IN+)
- R46 pad 1: +5V_ISO -> Net-(U19-IN+)
- R46 pad 2: Net-(Q7-S) -> GND_MCU
- R47 pad 1: Net-(D8-PadK) -> /MCU/MC_IU_SEN
- R47 pad 2: GND -> Net-(U18-IN-)
- R48 pad 1: +3V3 -> /MCU/MC_IV_SEN
- R48 pad 2: /MCU/~{BT_UBT} -> Net-(U19-IN-)
- R49 pad 1: PGND -> Net-(D17-PadK)
- R49 pad 2: Net-(U1-NW) -> GND_MCU
- R5 pad 1: Net-(D6-PadA) -> Net-(R4-Pad1)
- R5 pad 2: +5V -> AC1
- R50 pad 1: Net-(D9-A1) -> Net-(D18-PadK)
- R50 pad 2: /Inverter/MC_IDC_SEN_P -> GND_MCU
- R51 pad 1: Net-(D9-COM) -> /ENCODER/V_ENC
- R51 pad 2: /Inverter/MC_IDC_SEN_N -> /ENCODER/HOME
- R52 pad 1: Net-(U6-OUT) -> /ENCODER/V_ENC
- R52 pad 2: /MCU/MC_IDC_SEN -> /ENCODER/INDEX
- R53 pad 1: /Inverter/MC_UW -> /ENCODER/V_ENC
- R53 pad 2: Net-(R53-Pad2) -> /ENCODER/PULSE_B
- R54 pad 1: +3V3 -> /ENCODER/V_ENC
- R54 pad 2: /Inverter/MC_PWM_FLT -> /ENCODER/PULSE_A
- R55 pad 1: +24V_ISO -> +3V3_MCU
- R55 pad 2: /ENCODER/HOME -> /ENCODER/ENC_HOME
- R56 pad 1: Net-(R53-Pad2) -> +3V3_MCU
- R56 pad 2: Net-(R56-Pad2) -> /ENCODER/ENC_INDEX
- R57 pad 1: Net-(R56-Pad2) -> +3V3_MCU
- R57 pad 2: Net-(D16-COM) -> /ENCODER/ENC_B
- R58 pad 1: Net-(D16-COM) -> +3V3_MCU
- R58 pad 2: AGND -> /ENCODER/ENC_A
- R6 pad 1: /MCU/IND_ERR -> Net-(R4-Pad1)
- R6 pad 2: GND -> AC2
- R7 pad 1: /Inverter/IPM_PWM_FLT -> Net-(R4-Pad1)
- R7 pad 2: /Inverter/MC_PWM_FLT -> AC2
- R8 pad 1: /Inverter/MC_UU -> Net-(RL1-NC)
- R8 pad 2: Net-(R8-Pad2) -> PGND
- R9 pad 1: Net-(R8-Pad2) -> Net-(RL1-NC)
- R9 pad 2: Net-(R26-Pad1) -> PGND
- RL1 pad 1: Net-(Q10-D) -> Net-(RL1-COIL1)
- RL1 pad 2: +5V -> +12V_MCU
- RL1 pad 3: Net-(RL1-NC) -> Net-(RL2-NC)
- RL1 pad 4: Net-(RL1-NC) -> Net-(RL2-NC)
- RL1 pad 6: VDC -> Net-(BR1-DC+)
- RL2 pad 1: Net-(Q11-D) -> Net-(RL2-COIL1)
- RL2 pad 2: +5V -> +12V_MCU
- RL2 pad 3: Net-(RL1-NC) -> Net-(RL2-NC)
- RL2 pad 4: Net-(RL1-NC) -> Net-(RL2-NC)
- RL2 pad 6: Net-(BR1-DC+) -> VDC
- RV1 pad 1: AVDD -> +5V_INV
- RV1 pad 3: AGND -> GND_INV
- U1 pad 1: Net-(U1-VSU) -> Net-(U1-VFB)
- U1 pad 2: Net-(U1-VBU) -> Net-(U1-VCC)
- U1 pad 3: Net-(U1-VSV) -> Net-(U1-EN)
- U1 pad 4: Net-(U1-VBV) -> +24V_INV
- U1 pad 5: Net-(U1-VSW) -> GND_INV
- U1 pad 6: Net-(U1-VBW) -> Net-(U1-SW)
- U1 pad 7: /Inverter/IPM_PWM_UH -> Net-(U1-BOOST)
- U1 pad 8: /Inverter/IPM_PWM_VH -> GND_INV
- U1 pad 9: /Inverter/IPM_PWM_WH -> GND_INV
- U10 pad 1: Net-(U10-VFB) -> +3V3_MCU
- U10 pad 2: Net-(U10-VCC) -> /INVERTER/MC_PWM_WH
- U10 pad 3: Net-(U10-EN) -> /INVERTER/MC_PWM_WL
- U10 pad 4: +24V -> GND_MCU
- U10 pad 5: GND -> GND_INV
- U10 pad 6: Net-(U10-SW) -> /INVERTER/IPM_PWM_WL
- U10 pad 7: Net-(U10-BOOST) -> /INVERTER/IPM_PWM_WH
- U10 pad 8: GND -> +5V_INV
- U11 pad 1: /MCU/~{SRAM_CS} -> Net-(U11-IPP1)
- U11 pad 2: /MCU/SDI -> Net-(U11-IPP1)
- U11 pad 3: +3V3 -> /INVERTER/MC_U
- U11 pad 4: GND -> /INVERTER/MC_U
- U11 pad 5: /MCU/SDO -> GND_MCU
- U11 pad 6: /MCU/SCK -> Net-(U11-FILTER)
- U11 pad 7: +3V3 -> /INVERTER/MC_IU_HAL
- U11 pad 8: +3V3 -> +5V_MCU
- U12 pad 1: Net-(D3-COM) -> Net-(U12-IPP1)
- U12 pad 2: AGND -> Net-(U12-IPP1)
- U12 pad 3: Net-(U12-IN-) -> /INVERTER/MC_V
- U12 pad 4: Net-(U12-IN-) -> /INVERTER/MC_V
- U12 pad 5: AVDD -> GND_MCU
- U13 pad 1: +5V -> /INVERTER/IPM_TEMP_SEN
- U13 pad 2: +5V -> GND_INV
- U13 pad 3: +5V -> Net-(RV1-WIPER)
- U13 pad 4: GND -> /INVERTER/IPM_PWM_FLT
- U13 pad 5: unconnected-(U13-PWRGD-Pad5) -> +5V_INV
- U14 pad 1: Net-(U14-VFB) -> +5V_INV
- U14 pad 2: Net-(U14-VCC) -> Net-(D15-A1)
- U14 pad 3: Net-(U14-EN) -> Net-(D15-COM)
- U14 pad 4: +24V -> GND_INV
- U14 pad 5: GND -> GND_MCU
- U14 pad 6: Net-(U14-SW) -> Net-(U14-VOUT-)
- U14 pad 7: Net-(U14-BOOST) -> Net-(U14-VOUT+)
- U14 pad 8: GND -> +5V_MCU
- U15 pad 1: Net-(U1-U) -> +5V_INV
- U15 pad 2: Net-(U1-U) -> Net-(D16-A1)
- U15 pad 3: /Inverter/MC_UU -> Net-(D16-COM)
- U15 pad 4: /Inverter/MC_UU -> GND_INV
- U15 pad 5: GND -> GND_MCU
- U15 pad 6: Net-(U15-FILTER) -> Net-(U15-VOUT-)
- U15 pad 7: /Inverter/MC_IU_HAL -> Net-(U15-VOUT+)
- U15 pad 8: VREF -> +5V_MCU
- U16 pad 1: Net-(U1-V) -> GND_ADC
- U16 pad 2: Net-(U1-V) -> GND_MCU
- U16 pad 3: /Inverter/MC_UW -> +5V_MCU
- U16 pad 4: /Inverter/MC_UW -> Net-(U16-IN+)
- U16 pad 5: GND -> Net-(U16-IN-)
- U16 pad 6: Net-(U16-FILTER) -> Net-(U16-OUT)
- U17 pad 1: GND -> Net-(U17-IN+)
- U17 pad 2: +12V -> GND_MCU
- U17 pad 3: VREF -> Net-(U17-IN-)
- U18 pad 2: AGND -> GND_MCU
- U18 pad 5: AVDD -> +5V_MCU
- U19 pad 2: AGND -> GND_MCU
- U19 pad 5: AVDD -> +5V_MCU
- U2 pad 1: Net-(D2-COM) -> +5V_INV
- U2 pad 2: AGND -> GND_INV
- U2 pad 3: Net-(U2-IN-) -> +16V_INV
- U3 pad 1: GND -> Net-(U3-VFB)
- U3 pad 2: GND -> Net-(U3-VCC)
- U3 pad 3: VREF -> Net-(U3-EN)
- U3 pad 4: Net-(D5-A1) -> +24V_MCU
- U3 pad 5: Net-(D5-COM) -> GND_MCU
- U3 pad 6: Net-(U3-OUT) -> Net-(U3-SW)
- U4 pad 1: Net-(U4-VIN-) -> +5V_MCU
- U4 pad 2: AGND -> GND_MCU
- U4 pad 3: Net-(U4-VIN+) -> +12V_MCU
- U5 pad 1: GND -> +12V_MCU
- U5 pad 2: GND -> GND_MCU
- U5 pad 3: VREF -> +3V3_MCU
- U5 pad 4: Net-(D1-A1) -> GND_MCU
- U6 pad 1: GND -> +3V3_ADC
- U6 pad 2: GND -> GND_ADC
- U6 pad 3: VREF -> GND_MCU
- U6 pad 4: Net-(D9-A1) -> +5V_MCU
- U6 pad 5: Net-(D9-COM) -> GND_ADC
- U6 pad 6: Net-(U6-OUT) -> +5V_MCU
- U7 pad 1: Net-(D16-COM) -> Net-(U7-VSU)
- U7 pad 2: AGND -> Net-(U7-VBU)
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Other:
- board size 154 x 178.5 mm -> 159.9 x 155.6 mm

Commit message: V1 schematic update 18
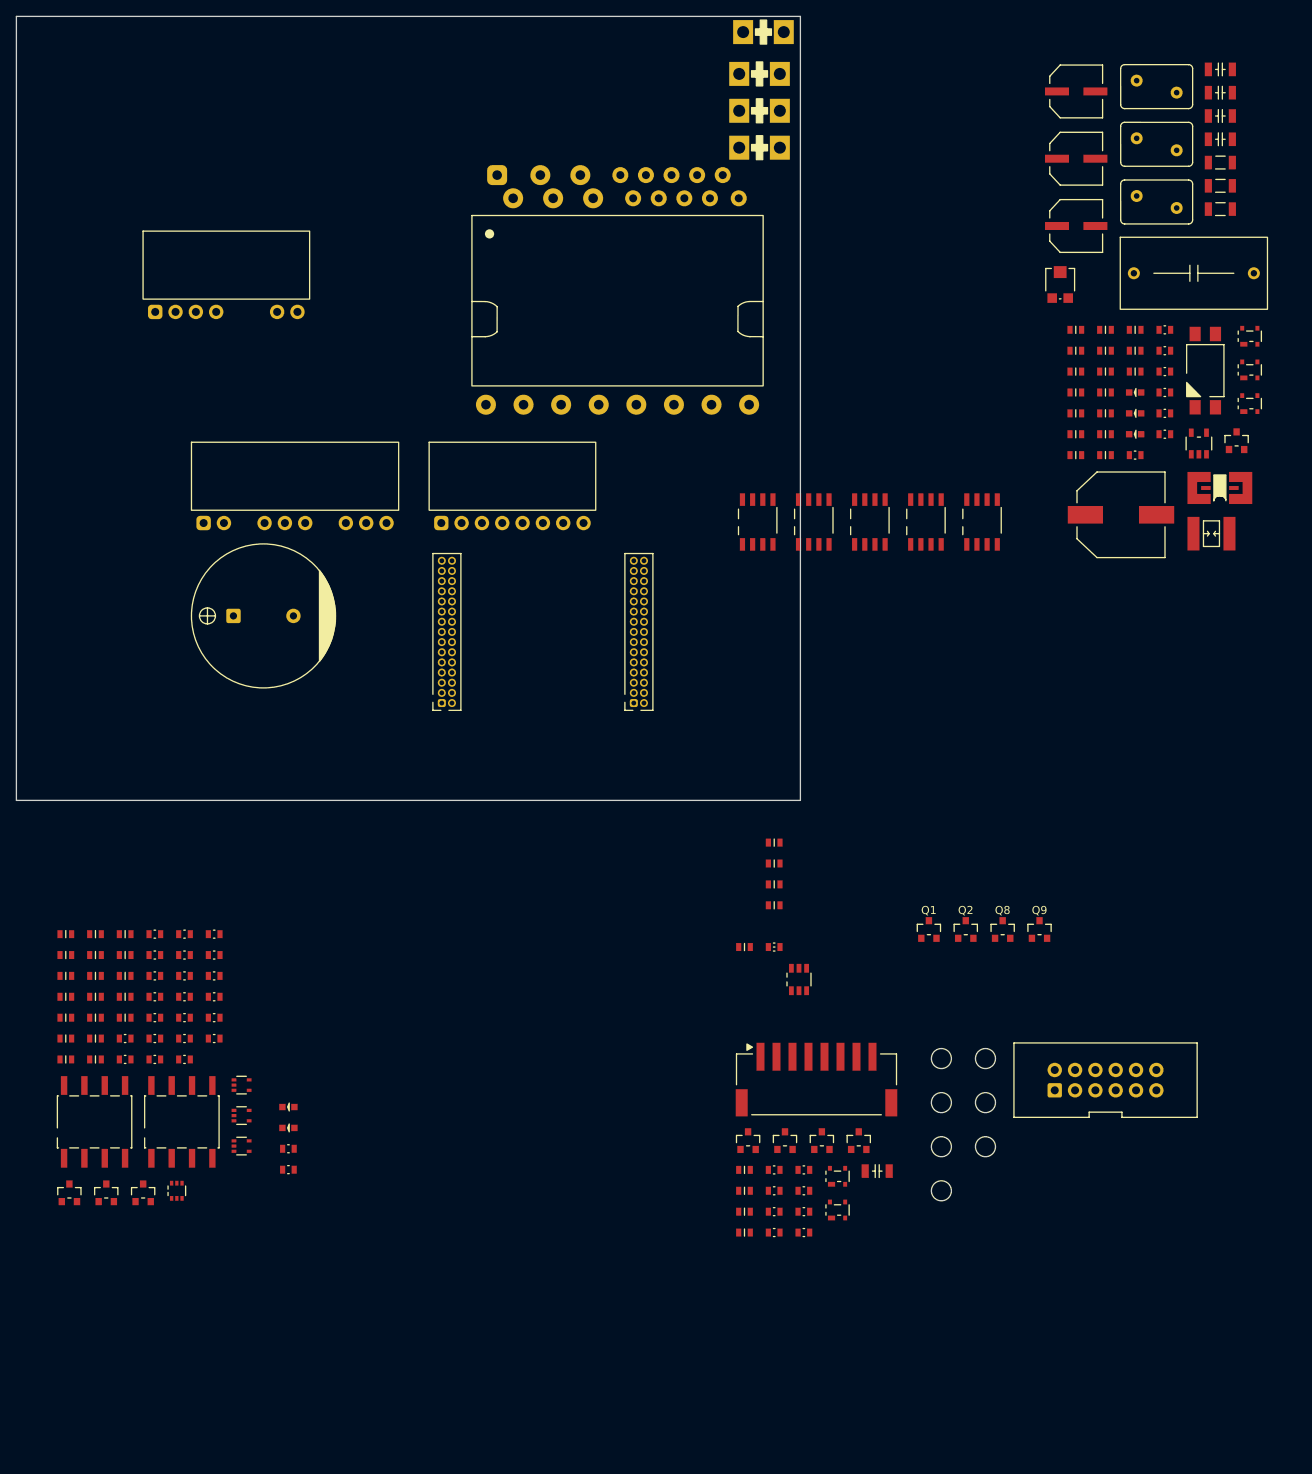
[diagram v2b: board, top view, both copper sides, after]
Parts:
- removed B1: 220V/50W, SAMPI:LAMP_6.35MM
- removed BR1: 400V/10A, SAMPI:GBJ25xx
- removed C1, C25: 470uF/35V, SAMPI:CAP_ELEC-10.3x10.3-DIA10
- removed C10, C22, C24, C26, C32, C4, C5: 100nF, SAMPI:CAP0603
- removed C11, C13, C16, C9: 100pF/2kV, SAMPI:CAP1206
- removed C12: 470uF/25V, SAMPI:CAP_ELEC-10.3x10.3-DIA10
- removed C14, C20, C3, C30: 10uF, SAMPI:CAP0603
- removed C15, C8: 1uF/400V, SAMPI:ECWFE2W105
- removed C17, C21, C7: 100nF/400V, SAMPI:CAP_FILM_6.0x12.0x12.5-P10
- removed C18: 680uF/450V, SAMPI:ESMQ451VSN681MA50S
- removed C19, C2, C28, C29: 10uF/35V, SAMPI:CAP1206
- removed C23, C6: 3.3nF, SAMPI:CAP0603
- removed C27: 470uF/16V, SAMPI:CAP_ELEC-8.3x8.3-DIA8.0
- removed C34: 220uF/6.3V, SAMPI:CAP1411
- removed D1, D6: 24V, SAMPI:DO-214AA-12
- removed D2, D5: 75V/150mA, SAMPI:SOD-323
- removed D3, D4: 6V2, SAMPI:SOD80C-LL34
- removed D7: PWR, SAMPI:LED0603
- removed FT1, FT4: 15mH/500mA, SAMPI:EE8.3
- removed FT2: 5mH/2.5A, SAMPI:IND-SQ1010
- removed FT3: 120R@100MHz, SAMPI:FT0603
- removed G1: 300V, SAMPI:GDT1812_3532
- removed L1: 68uH/1A, SAMPI:IND-8D43-8045
- removed L2: 56uH/1A, SAMPI:IND-8D43-8045
- removed M1, M2, M3, M4: 470V/1.2kA, SAMPI:MOV5MM
- removed MD1: 24V±2%/3W, SAMPI:HLK-PMxx
- removed MD2: 24V±2%/10W, SAMPI:HLK-10M
- removed R1, R10, R11, R12: 10K, SAMPI:RES0603
- removed R13: 140K, 1%, SAMPI:RES0603
- removed R14, R3: 10K, 1%, SAMPI:RES0603
- removed R15: 1K, SAMPI:RES0603
- removed R2: 191K, 1%, SAMPI:RES0603
- removed R4, R5, R6, R7, R8, R9: 1M, SAMPI:RES1206
- removed RL1, RL2: 5V/30A, SAMPI:SLA-12VDC-SL-C
- removed U1: SMPS 16V±2%/0.6A, SAMPI:TDFN8_2x3_MCHP
- removed U2, U4: LDO 5V±1%, SAMPI:SOT-89
- removed U3: SMPS 12V±2%/0.8A, SAMPI:TDFN8_2x3_MCHP
- removed U5: LDO 3V3±2%, SAMPI:SOT-223-3
- added C88: 100uF/450V, SAMPI:CAP_ELEC-18.0x51.5-LS7.5, F.Cu at (45.5, 88.8)
- added J14: MCU PWR, SAMPI:HDM1x8x2.54_TH_RA, F.Cu at (76.6, 77.2)
- added J15: INV PWR & RELAYS, SAMPI:HDM1x8x2.54_TH_RA, F.Cu at (40.8, 50.8)
- added J16: HIGH VOLTAGE OUTPUTS, SAMPI:HDF1x10x2.54_TH_RA, F.Cu at (49.4, 77.2)
- added J2: U, SAMPI:QC-6.3, F.Cu at (107.5, 21.1)
- added Q8: 60V/265mA, SAMPI:SOT23, F.Cu at (137.9, 128.0)
- added Q9: 60V/265mA, SAMPI:SOT23, F.Cu at (142.5, 128.0)
- J3: value AC POWER INPUT -> V; footprint SAMPI:TMB3_9.5 -> SAMPI:QC-6.3
- J4: value FAN -> W; footprint SAMPI:HDM-2x2.54-TH -> SAMPI:QC-6.3
- J5: value MOTOR -> N; footprint SAMPI:TMB4_9.5 -> SAMPI:QC-6.3
- Q1, Q2: value 20V/1A -> 60V/265mA
- moved J4 106.1 mm to (107.5, 30.3)
- moved Q1 54.7 mm to (128.7, 128.0)
- moved Q2 54.7 mm to (133.3, 128.0)
- moved MD3 50.2 mm to (80.4, 90.8)
- moved J5 45.8 mm to (108.0, 15.8)
- moved J3 35.9 mm to (107.5, 25.7)
- moved U7 35.7 mm to (89.7, 48.1)
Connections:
- J3 pad 1: CHASSIS -> /INVERTER/MC_V
- J4 pad 1: +12V_MCU -> /INVERTER/MC_W
- MD3 pad L10: /INVERTER POWER/~{DEV_RELAY} -> /MCU POWER/~{DEV_RELAY}
- MD3 pad L9: /INVERTER POWER/PWR_RELAY -> /MCU POWER/PWR_RELAY
- Q1 pad 1: /INVERTER POWER/PWR_RELAY -> /ENCODER/V_ENC
- Q1 pad 2: GND_MCU -> /ENCODER/PULSE_A
- Q2 pad 1: /INVERTER POWER/~{DEV_RELAY} -> /ENCODER/V_ENC
- Q2 pad 2: GND_MCU -> /ENCODER/PULSE_B
- Q4 pad 3: /ENCODER/HOME -> Net-(Q4-D)
- Q5 pad 3: /ENCODER/INDEX -> Net-(Q5-D)
- Q6 pad 3: /ENCODER/PULSE_B -> Net-(Q2-D)
- Q7 pad 3: /ENCODER/PULSE_A -> Net-(Q1-D)
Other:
- board size 159.9 x 155.6 mm -> 98 x 98 mm
